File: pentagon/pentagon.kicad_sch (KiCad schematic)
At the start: 28 parts, among them J1 Conn_01x05_Pin, J2 Conn_01x05_Pin, J3 Conn_01x05_Pin, J4 Conn_01x05_Pin, J5 Conn_01x05_Pin

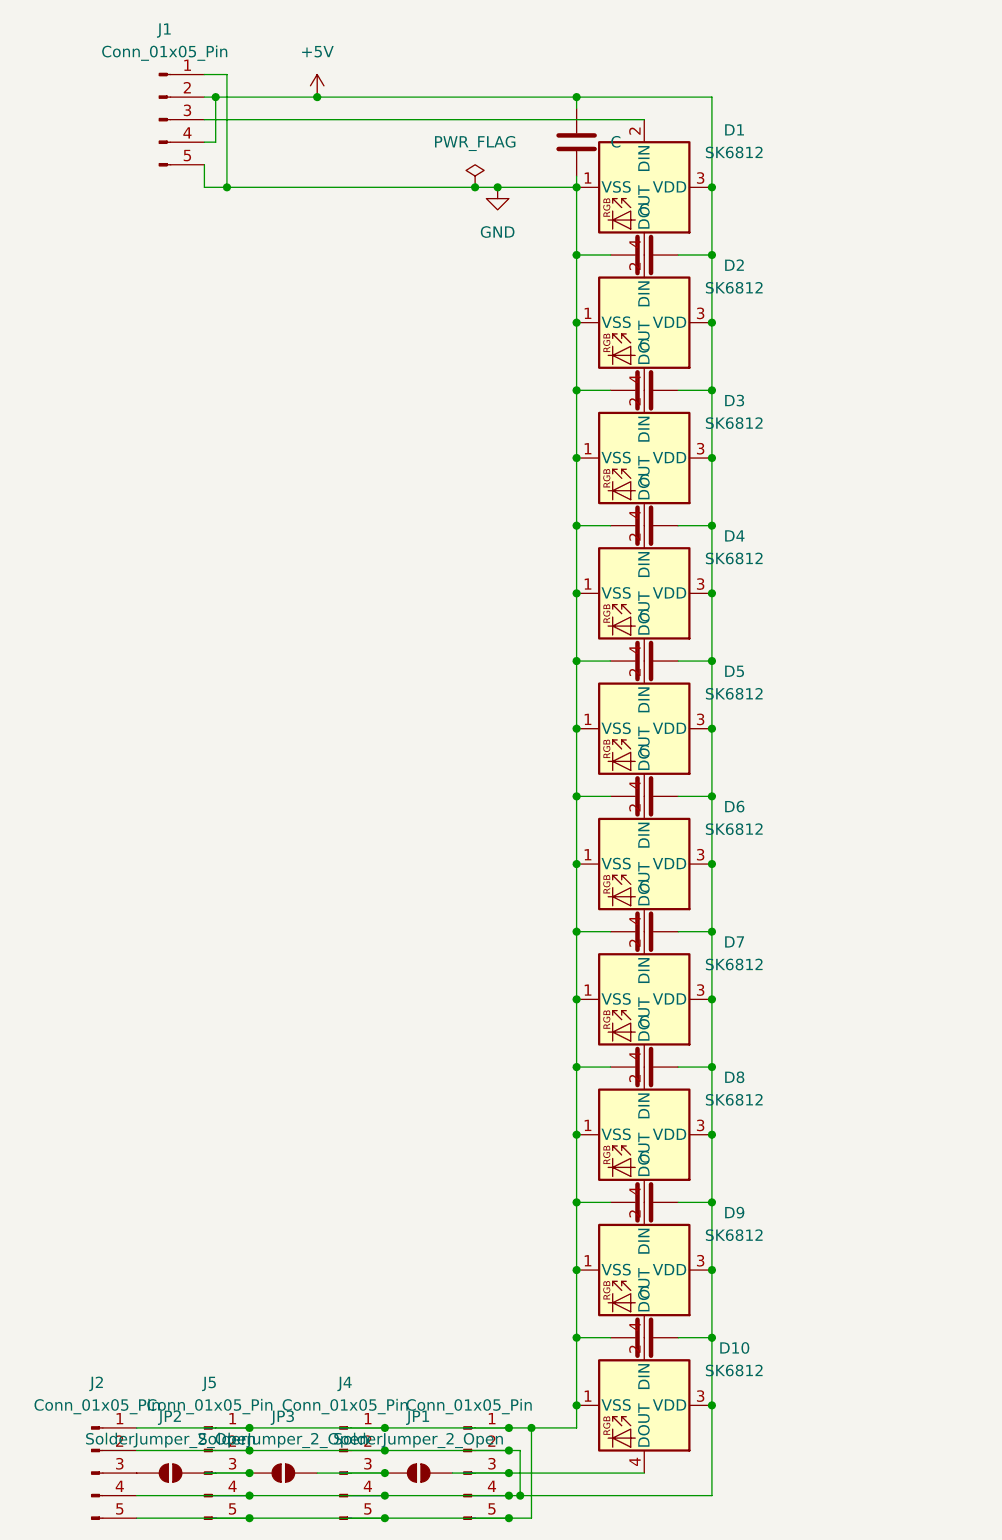
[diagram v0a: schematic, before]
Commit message: updated all coolness
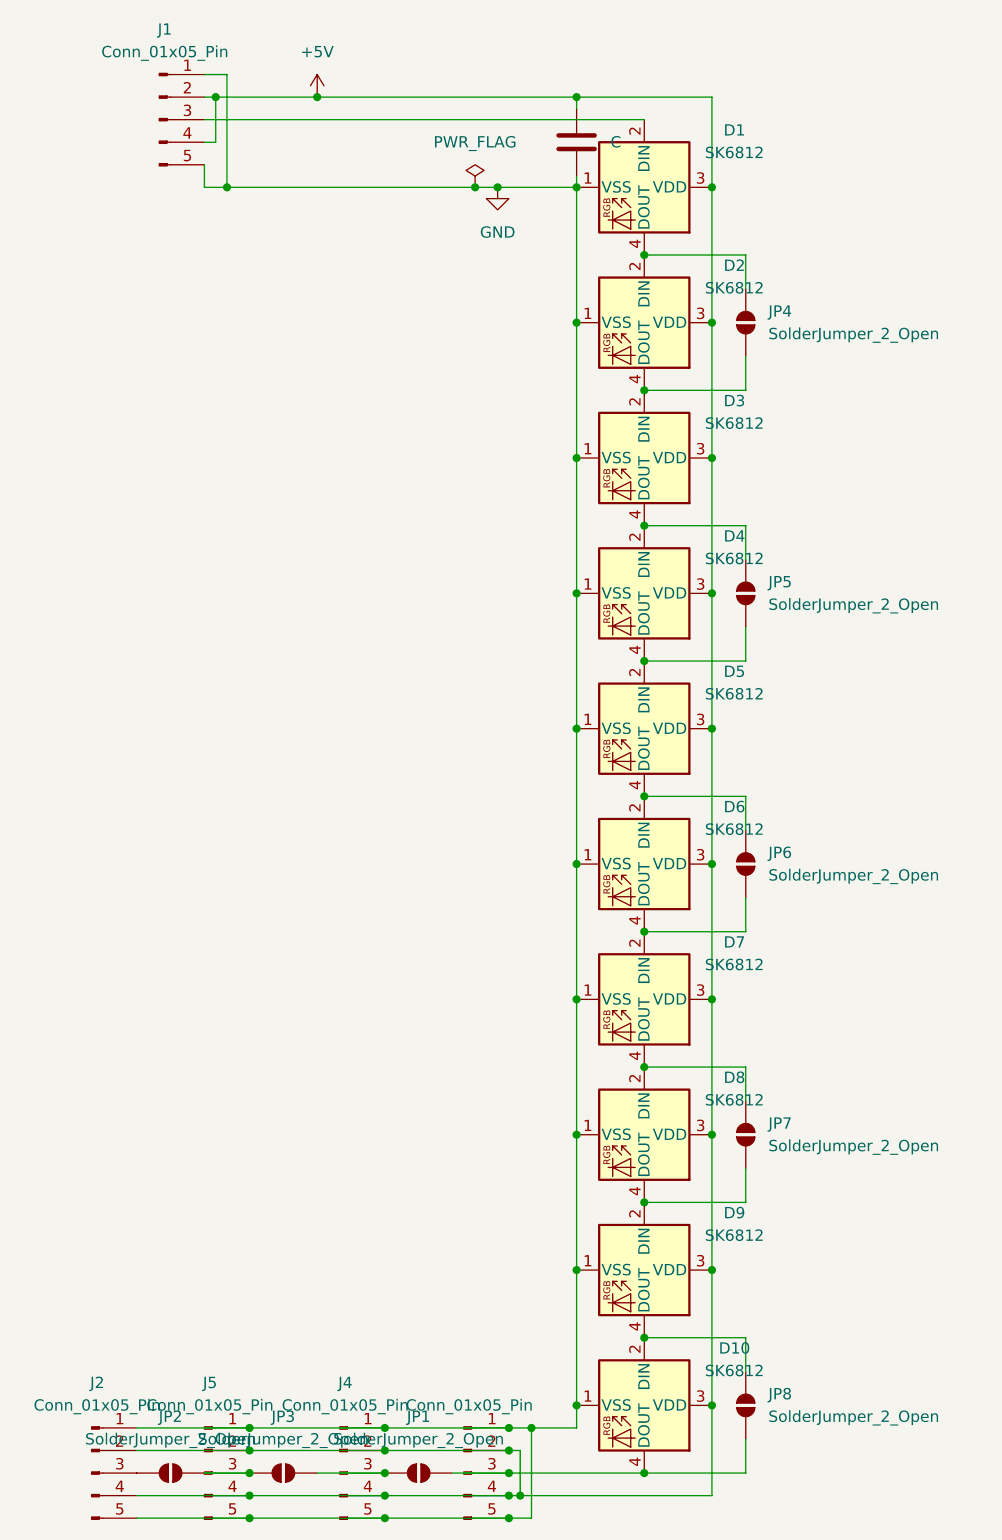
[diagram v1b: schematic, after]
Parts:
- removed C10, C2, C3, C4, C5, C6, C7, C8, C9: C, Capacitor_SMD:C_0805_2012Metric_Pad1.18x1.45mm_HandSolder, symbol Device:C
- added JP4, JP5, JP6, JP7, JP8: SolderJumper_2_Open, Jumper:SolderJumper-2_P1.3mm_Open_RoundedPad1.0x1.5mm, symbol Jumper:SolderJumper_2_Open
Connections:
- net at D6.4 (DOUT), D7.2 (DIN): now also JP6.1 (A)
- net at D7.4 (DOUT), D8.2 (DIN): now also JP7.2 (B)
- net at D3.4 (DOUT), D4.2 (DIN): now also JP5.2 (B)
- net at D4.4 (DOUT), D5.2 (DIN): now also JP5.1 (A)
- net at D8.4 (DOUT), D9.2 (DIN): now also JP7.1 (A)
- net at D10.2 (DIN), D9.4 (DOUT): now also JP8.2 (B)
- net at D10.4 (DOUT), J3.3 (Pin_3), JP1.2 (B): now also JP8.1 (A)
- net at D1.4 (DOUT), D2.2 (DIN): now also JP4.2 (B)
- net at D2.4 (DOUT), D3.2 (DIN): now also JP4.1 (A)
- net at D5.4 (DOUT), D6.2 (DIN): now also JP6.2 (B)
